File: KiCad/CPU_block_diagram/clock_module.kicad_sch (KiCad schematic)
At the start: 17 parts, among them U1 74LS04, U2 LM555xN, U3 74LS08, U4 74LS32, U5 LM555xN, U6 LM555xN

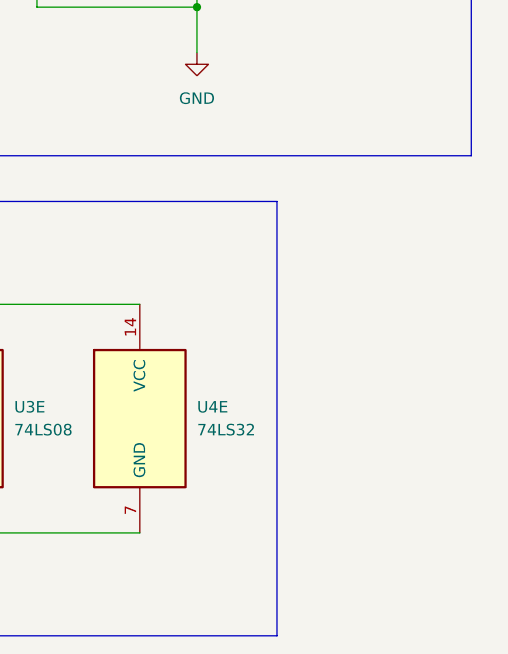
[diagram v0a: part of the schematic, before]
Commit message: vault backup: 2026-01-03 05:38:52
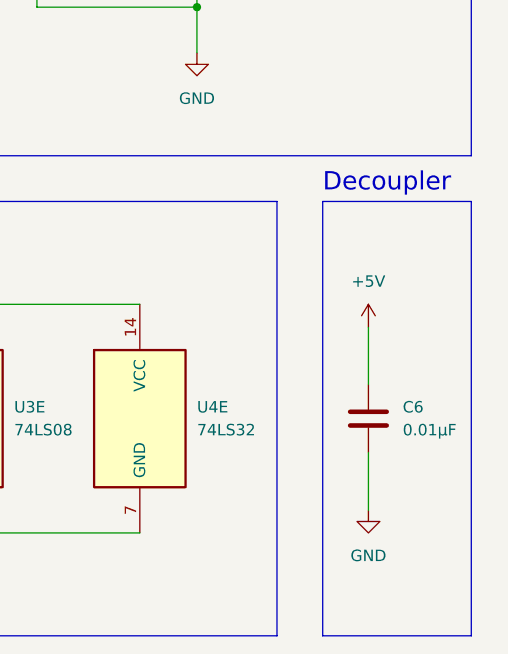
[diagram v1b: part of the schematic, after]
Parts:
- added C6: 0.01µF, symbol Device:C
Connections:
- net +5V: now also C6.1
- net GND: now also C6.2
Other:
- note added: "Decoupler"
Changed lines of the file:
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@@
+	)
+	(rectangle
+		(start 252.73 87.63)
+		(end 269.24 135.89)
+		(stroke
+			(width 0)
+			(type default)
+		)
+		(fill
+			(type none)
+		)
 	)
 	(rectangle
@@
 		(fill
 			(type none)
+		)
+	)
+	(text "Decoupler"
+		(exclude_from_sim no)
+		(at 252.73 85.598 0)
+		(effects
+			(font
+				(size 2.032 2.032)
+			)
+			(justify left)
 		)
 	)
@@
 	(wire
 		(pts
+			(xy 257.81 101.6) (xy 257.81 107.95)
+		)
+		(stroke
+			(width 0)
+			(type default)
+		)
+	)
+	(wire
+		(pts
 			(xy 217.17 38.1) (xy 241.3 38.1)
 		)
@@
 		(pts
 			(xy 220.98 55.88) (xy 228.6 55.88)
+		)
+		(stroke
+			(width 0)
+			(type default)
+		)
+	)
+	(wire
+		(pts
+			(xy 257.81 121.92) (xy 257.81 115.57)
 		)
 		(stroke
@@
 	)
 	(symbol
+		(lib_id "power:GND")
+		(at 257.81 121.92 0)
+		(unit 1)
+		(exclude_from_sim no)
+		(in_bom yes)
+		(on_board yes)
+		(dnp no)
+		(fields_autoplaced yes)
+		(property "Reference" "#PWR015"
+			(at 257.81 128.27 0)
+			(effects
+				(font
+					(size 1.27 1.27)
+				)
+				(hide yes)
+			)
+		)
+		(property "Value" "GND"
+			(at 257.81 127 0)
+			(effects
+				(font
+					(size 1.27 1.27)
+				)
+			)
+		)
+		(property "Footprint" ""
+			(at 257.81 121.92 0)
+			(effects
+				(font
+					(size 1.27 1.27)
+				)
+				(hide yes)
+			)
+		)
+		(property "Datasheet" ""
+			(at 257.81 121.92 0)
+			(effects
+				(font
+					(size 1.27 1.27)
+				)
+				(hide yes)
+			)
+		)
+		(property "Description" "Power symbol creates a global label with name \"GND\" , ground"
+			(at 257.81 121.92 0)
+			(effects
+				(font
+					(size 1.27 1.27)
+				)
+				(hide yes)
+			)
+		)
+		(pin "1"
+		)
+		(instances
+			(project ""
+				(path "/5324683e-15fd-4fa9-8f28-7726564ef1dc/23156860-93e6-4eb1-8f6c-79601c8beb45"
+					(reference "#PWR015")
+					(unit 1)
+				)
+			)
+		)
+	)
+	(symbol
 		(lib_id "Timer:LM555xN")
 		(at 76.2 53.34 0)
@@
 	)
 	(symbol
+		(lib_id "power:+5V")
+		(at 257.81 101.6 0)
+		(unit 1)
+		(exclude_from_sim no)
+		(in_bom yes)
+		(on_board yes)
+		(dnp no)
+		(fields_autoplaced yes)
+		(property "Reference" "#PWR014"
+			(at 257.81 105.41 0)
+			(effects
+				(font
+					(size 1.27 1.27)
+				)
+				(hide yes)
+			)
+		)
+		(property "Value" "+5V"
+			(at 257.81 96.52 0)
+			(effects
+				(font
+					(size 1.27 1.27)
+				)
+			)
+		)
+		(property "Footprint" ""
+			(at 257.81 101.6 0)
+			(effects
+				(font
+					(size 1.27 1.27)
+				)
+				(hide yes)
+			)
+		)
+		(property "Datasheet" ""
+			(at 257.81 101.6 0)
+			(effects
+				(font
+					(size 1.27 1.27)
+				)
+				(hide yes)
+			)
+		)
+		(property "Description" "Power symbol creates a global label with name \"+5V\""
+			(at 257.81 101.6 0)
+			(effects
+				(font
+					(size 1.27 1.27)
+				)
+				(hide yes)
+			)
+		)
+		(pin "1"
+		)
+		(instances
+			(project ""
+				(path "/5324683e-15fd-4fa9-8f28-7726564ef1dc/23156860-93e6-4eb1-8f6c-79601c8beb45"
+					(reference "#PWR014")
+					(unit 1)
+				)
+			)
+		)
+	)
+	(symbol
 		(lib_id "Timer:LM555xN")
 		(at 238.76 53.34 0)
@@
 					(unit 1)
 				)
+			)
+		)
+	)
+	(symbol
+		(lib_id "Device:C")
+		(at 257.81 111.76 0)
+		(unit 1)
+		(exclude_from_sim no)
+		(in_bom yes)
+		(on_board yes)
+		(dnp no)
+		(fields_autoplaced yes)
+		(property "Reference" "C6"
+			(at 261.62 110.4899 0)
+			(effects
+				(font
+					(size 1.27 1.27)
+				)
+				(justify left)
+			)
+		)
+		(property "Value" "0.01µF"
+			(at 261.62 113.0299 0)
+			(effects
+				(font
+					(size 1.27 1.27)
+				)
+				(justify left)
+			)
+		)
+		(property "Footprint" ""
+			(at 258.7752 115.57 0)
+			(effects
+				(font
+					(size 1.27 1.27)
+				)
+				(hide yes)
+			)
+		)
+		(property "Datasheet" "~"
+			(at 257.81 111.76 0)
+			(effects
+				(font
+					(size 1.27 1.27)
+				)
+				(hide yes)
+			)
+		)
+		(property "Description" "Unpolarized capacitor"
+			(at 257.81 111.76 0)
+			(effects
+				(font
+					(size 1.27 1.27)
+				)
+				(hide yes)
+			)
+		)
+		(pin "2"
+		)
+		(pin "1"
+		)
+		(instances
+			(project ""
+				(path "/5324683e-15fd-4fa9-8f28-7726564ef1dc/23156860-93e6-4eb1-8f6c-79601c8beb45"
+					(reference "C6")
+					(unit 1)
+				)

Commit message: vault backup: 2026-01-03 11:53:08
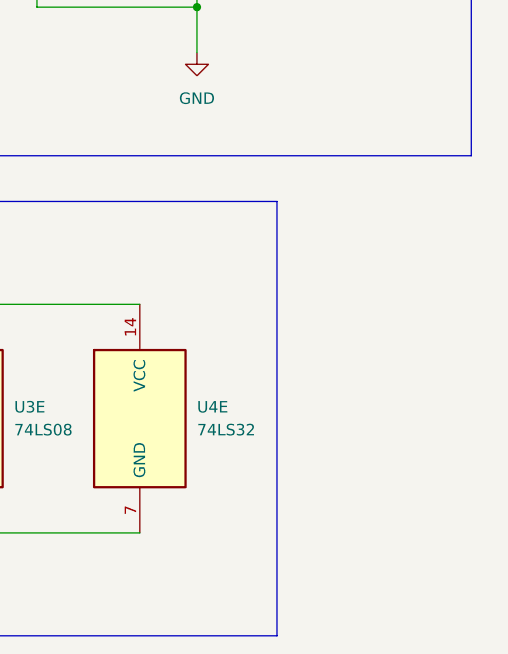
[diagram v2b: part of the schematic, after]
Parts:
- removed C6: 0.01µF, symbol Device:C
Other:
- note removed: "Decoupler"
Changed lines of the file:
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@@
-	)
-	(rectangle
-		(start 252.73 87.63)
-		(end 269.24 135.89)
-		(stroke
-			(width 0)
-			(type default)
-		)
-		(fill
-			(type none)
-		)
 	)
 	(rectangle
@@
 		(fill
 			(type none)
-		)
-	)
-	(text "Decoupler"
-		(exclude_from_sim no)
-		(at 252.73 85.598 0)
-		(effects
-			(font
-				(size 2.032 2.032)
-			)
-			(justify left)
 		)
 	)
@@
 	(wire
 		(pts
-			(xy 257.81 101.6) (xy 257.81 107.95)
-		)
-		(stroke
-			(width 0)
-			(type default)
-		)
-	)
-	(wire
-		(pts
 			(xy 217.17 38.1) (xy 241.3 38.1)
 		)
@@
 		(pts
 			(xy 220.98 55.88) (xy 228.6 55.88)
-		)
-		(stroke
-			(width 0)
-			(type default)
-		)
-	)
-	(wire
-		(pts
-			(xy 257.81 121.92) (xy 257.81 115.57)
 		)
 		(stroke
@@
 	)
 	(symbol
-		(lib_id "power:GND")
-		(at 257.81 121.92 0)
-		(unit 1)
-		(exclude_from_sim no)
-		(in_bom yes)
-		(on_board yes)
-		(dnp no)
-		(fields_autoplaced yes)
-		(property "Reference" "#PWR015"
-			(at 257.81 128.27 0)
-			(effects
-				(font
-					(size 1.27 1.27)
-				)
-				(hide yes)
-			)
-		)
-		(property "Value" "GND"
-			(at 257.81 127 0)
-			(effects
-				(font
-					(size 1.27 1.27)
-				)
-			)
-		)
-		(property "Footprint" ""
-			(at 257.81 121.92 0)
-			(effects
-				(font
-					(size 1.27 1.27)
-				)
-				(hide yes)
-			)
-		)
-		(property "Datasheet" ""
-			(at 257.81 121.92 0)
-			(effects
-				(font
-					(size 1.27 1.27)
-				)
-				(hide yes)
-			)
-		)
-		(property "Description" "Power symbol creates a global label with name \"GND\" , ground"
-			(at 257.81 121.92 0)
-			(effects
-				(font
-					(size 1.27 1.27)
-				)
-				(hide yes)
-			)
-		)
-		(pin "1"
-		)
-		(instances
-			(project ""
-				(path "/5324683e-15fd-4fa9-8f28-7726564ef1dc/23156860-93e6-4eb1-8f6c-79601c8beb45"
-					(reference "#PWR015")
-					(unit 1)
-				)
-			)
-		)
-	)
-	(symbol
 		(lib_id "Timer:LM555xN")
 		(at 76.2 53.34 0)
@@
 	)
 	(symbol
-		(lib_id "power:+5V")
-		(at 257.81 101.6 0)
-		(unit 1)
-		(exclude_from_sim no)
-		(in_bom yes)
-		(on_board yes)
-		(dnp no)
-		(fields_autoplaced yes)
-		(property "Reference" "#PWR014"
-			(at 257.81 105.41 0)
-			(effects
-				(font
-					(size 1.27 1.27)
-				)
-				(hide yes)
-			)
-		)
-		(property "Value" "+5V"
-			(at 257.81 96.52 0)
-			(effects
-				(font
-					(size 1.27 1.27)
-				)
-			)
-		)
-		(property "Footprint" ""
-			(at 257.81 101.6 0)
-			(effects
-				(font
-					(size 1.27 1.27)
-				)
-				(hide yes)
-			)
-		)
-		(property "Datasheet" ""
-			(at 257.81 101.6 0)
-			(effects
-				(font
-					(size 1.27 1.27)
-				)
-				(hide yes)
-			)
-		)
-		(property "Description" "Power symbol creates a global label with name \"+5V\""
-			(at 257.81 101.6 0)
-			(effects
-				(font
-					(size 1.27 1.27)
-				)
-				(hide yes)
-			)
-		)
-		(pin "1"
-		)
-		(instances
-			(project ""
-				(path "/5324683e-15fd-4fa9-8f28-7726564ef1dc/23156860-93e6-4eb1-8f6c-79601c8beb45"
-					(reference "#PWR014")
-					(unit 1)
-				)
-			)
-		)
-	)
-	(symbol
 		(lib_id "Timer:LM555xN")
 		(at 238.76 53.34 0)
@@
 					(unit 1)
 				)
-			)
-		)
-	)
-	(symbol
-		(lib_id "Device:C")
-		(at 257.81 111.76 0)
-		(unit 1)
-		(exclude_from_sim no)
-		(in_bom yes)
-		(on_board yes)
-		(dnp no)
-		(fields_autoplaced yes)
-		(property "Reference" "C6"
-			(at 261.62 110.4899 0)
-			(effects
-				(font
-					(size 1.27 1.27)
-				)
-				(justify left)
-			)
-		)
-		(property "Value" "0.01µF"
-			(at 261.62 113.0299 0)
-			(effects
-				(font
-					(size 1.27 1.27)
-				)
-				(justify left)
-			)
-		)
-		(property "Footprint" ""
-			(at 258.7752 115.57 0)
-			(effects
-				(font
-					(size 1.27 1.27)
-				)
-				(hide yes)
-			)
-		)
-		(property "Datasheet" "~"
-			(at 257.81 111.76 0)
-			(effects
-				(font
-					(size 1.27 1.27)
-				)
-				(hide yes)
-			)
-		)
-		(property "Description" "Unpolarized capacitor"
-			(at 257.81 111.76 0)
-			(effects
-				(font
-					(size 1.27 1.27)
-				)
-				(hide yes)
-			)
-		)
-		(pin "2"
-		)
-		(pin "1"
-		)
-		(instances
-			(project ""
-				(path "/5324683e-15fd-4fa9-8f28-7726564ef1dc/23156860-93e6-4eb1-8f6c-79601c8beb45"
-					(reference "C6")
-					(unit 1)
-				)
